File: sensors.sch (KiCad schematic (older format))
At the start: 16 parts, among them U4 MPU-9250, U5 MS5611-01BA, U6 VL6180X

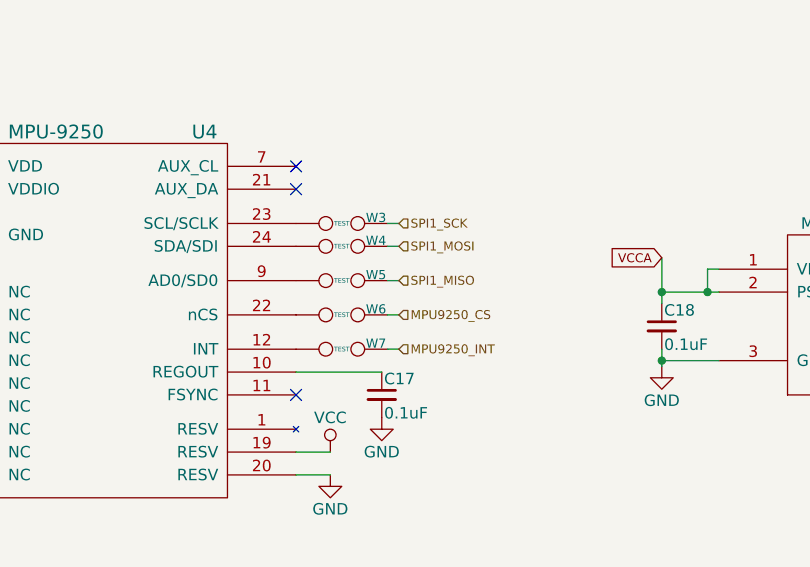
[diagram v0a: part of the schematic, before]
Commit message: Regenerate netlist & Start placing footprints
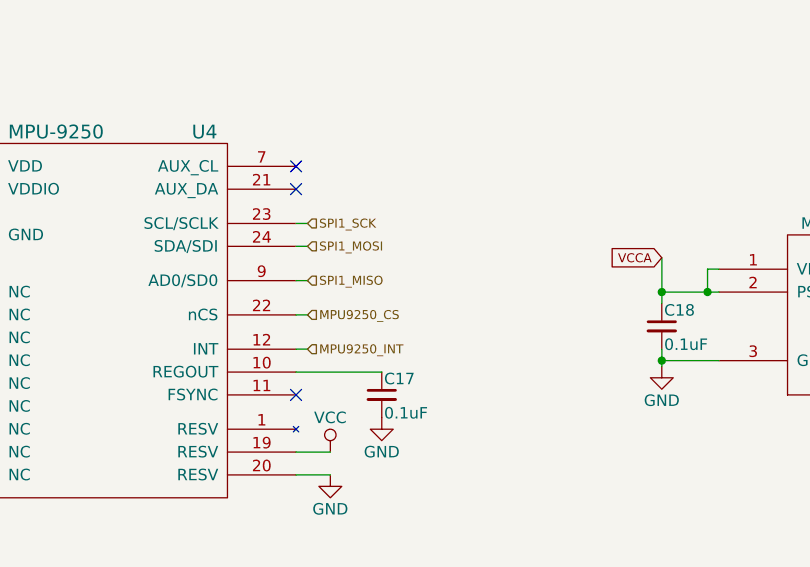
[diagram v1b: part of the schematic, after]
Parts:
- removed W3, W4, W5, W6, W7: TEST, _std:Measurement_Point_Round-SMD-Pad_Small, symbol TEST
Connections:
- net MPU9250_CS: now also U4.22 (nCS)
- net MPU9250_INT: now also U4.12 (INT)
- net SPI1_MISO: now also U4.9 (AD0/SD0)
- net SPI1_MOSI: now also U4.24 (SDA/SDI)
- net SPI1_SCK: now also U4.23 (SCL/SCLK)
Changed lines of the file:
@@
 EESchema Schematic File Version 2
-LIBS:speedy-rescue
 LIBS:speedy-cache
 LIBS:power
@@
 	1    0    0    -1
 $EndComp
-Text HLabel 3825 2125 2    39   Input ~ 0
+Text HLabel 3425 2125 2    39   Input ~ 0
 SPI1_SCK
-Text HLabel 3825 2225 2    39   Input ~ 0
+Text HLabel 3425 2225 2    39   Input ~ 0
 SPI1_MOSI
-Text HLabel 3825 2375 2    39   Input ~ 0
+Text HLabel 3425 2375 2    39   Input ~ 0
 SPI1_MISO
-Text HLabel 3825 2525 2    39   Input ~ 0
+Text HLabel 3425 2525 2    39   Input ~ 0
 MPU9250_CS
-Text HLabel 3825 2675 2    39   Input ~ 0
+Text HLabel 3425 2675 2    39   Input ~ 0
 MPU9250_INT
 $Comp
@@
 	3750 2775 3375 2775
 Wire Wire Line
-	3825 2375 3775 2375
-Wire Wire Line
-	3825 2525 3775 2525
-Wire Wire Line
-	3825 2225 3775 2225
-Wire Wire Line
-	3825 2125 3775 2125
-Wire Wire Line
-	3825 2675 3775 2675
+	3425 2375 3375 2375
+Wire Wire Line
+	3425 2525 3375 2525
+Wire Wire Line
+	3425 2225 3375 2225
+Wire Wire Line
+	3425 2125 3375 2125
+Wire Wire Line
+	3425 2675 3375 2675
 Wire Wire Line
 	3525 3225 3375 3225
@@
 Text GLabel 10275 1950 2    39   Input ~ 0
 VCCA
-$Comp
-L TEST W3
-U 1 1 55799AAF
-P 3575 2125
-F 0 "W3" H 3725 2150 40  0000 C CNN
-F 1 "TEST" H 3575 2125 20  0000 C CNN
-F 2 "_std:Measurement_Point_Round-SMD-Pad_Small" H 3575 2125 60  0001 C CNN
-F 3 "" H 3575 2125 60  0000 C CNN
-	1    3575 2125
-	1    0    0    -1
-$EndComp
-$Comp
-L TEST W4
-U 1 1 55799BD9
-P 3575 2225
-F 0 "W4" H 3725 2250 40  0000 C CNN
-F 1 "TEST" H 3575 2225 20  0000 C CNN
-F 2 "_std:Measurement_Point_Round-SMD-Pad_Small" H 3575 2225 60  0001 C CNN
-F 3 "" H 3575 2225 60  0000 C CNN
-	1    3575 2225
-	1    0    0    -1
-$EndComp
-$Comp
-L TEST W5
-U 1 1 55799C09
-P 3575 2375
-F 0 "W5" H 3725 2400 40  0000 C CNN
-F 1 "TEST" H 3575 2375 20  0000 C CNN
-F 2 "_std:Measurement_Point_Round-SMD-Pad_Small" H 3575 2375 60  0001 C CNN
-F 3 "" H 3575 2375 60  0000 C CNN
-	1    3575 2375
-	1    0    0    -1
-$EndComp
-$Comp
-L TEST W6
-U 1 1 55799C3F
-P 3575 2525
-F 0 "W6" H 3725 2550 40  0000 C CNN
-F 1 "TEST" H 3575 2525 20  0000 C CNN
-F 2 "_std:Measurement_Point_Round-SMD-Pad_Small" H 3575 2525 60  0001 C CNN
-F 3 "" H 3575 2525 60  0000 C CNN
-	1    3575 2525
-	1    0    0    -1
-$EndComp
-$Comp
-L TEST W7
-U 1 1 55799C79
-P 3575 2675
-F 0 "W7" H 3725 2700 40  0000 C CNN
-F 1 "TEST" H 3575 2675 20  0000 C CNN
-F 2 "_std:Measurement_Point_Round-SMD-Pad_Small" H 3575 2675 60  0001 C CNN
-F 3 "" H 3575 2675 60  0000 C CNN
-	1    3575 2675
-	1    0    0    -1
-$EndComp
 Wire Notes Line
 	475  4075 11225 4075
